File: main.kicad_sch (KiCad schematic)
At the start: 124 parts, among them SW1 SW_Push

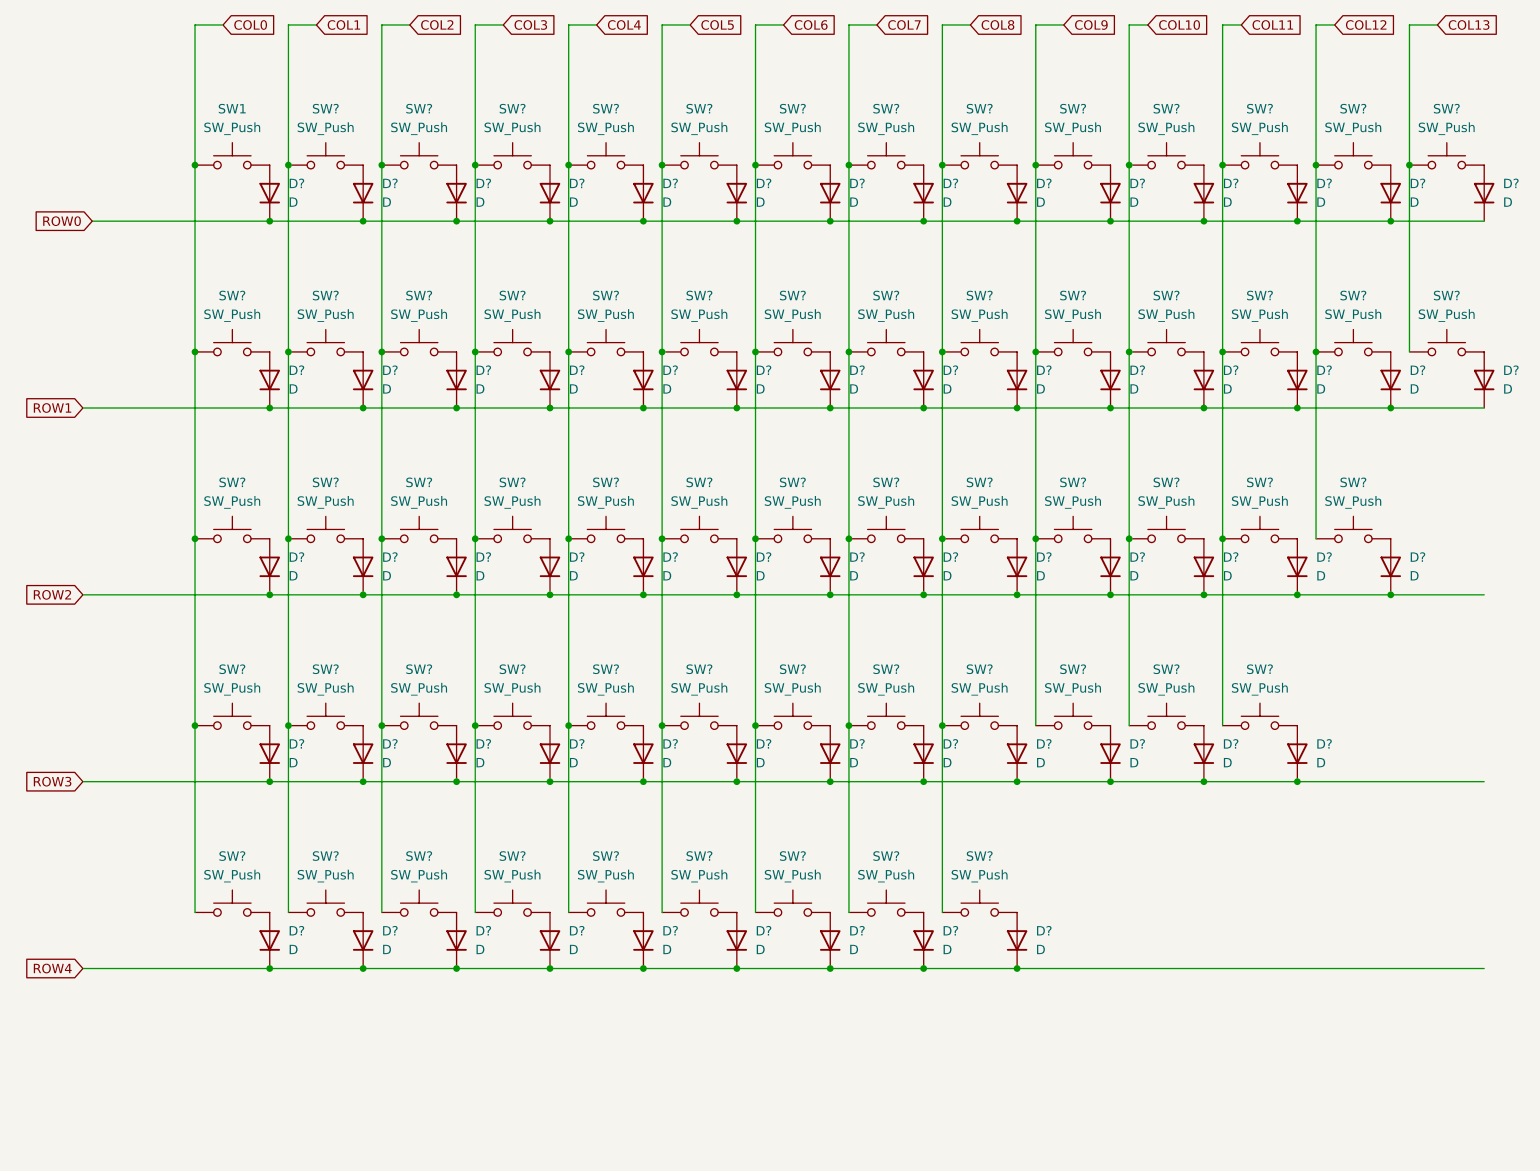
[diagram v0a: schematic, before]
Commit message: Finalilize the Keybord Shematic
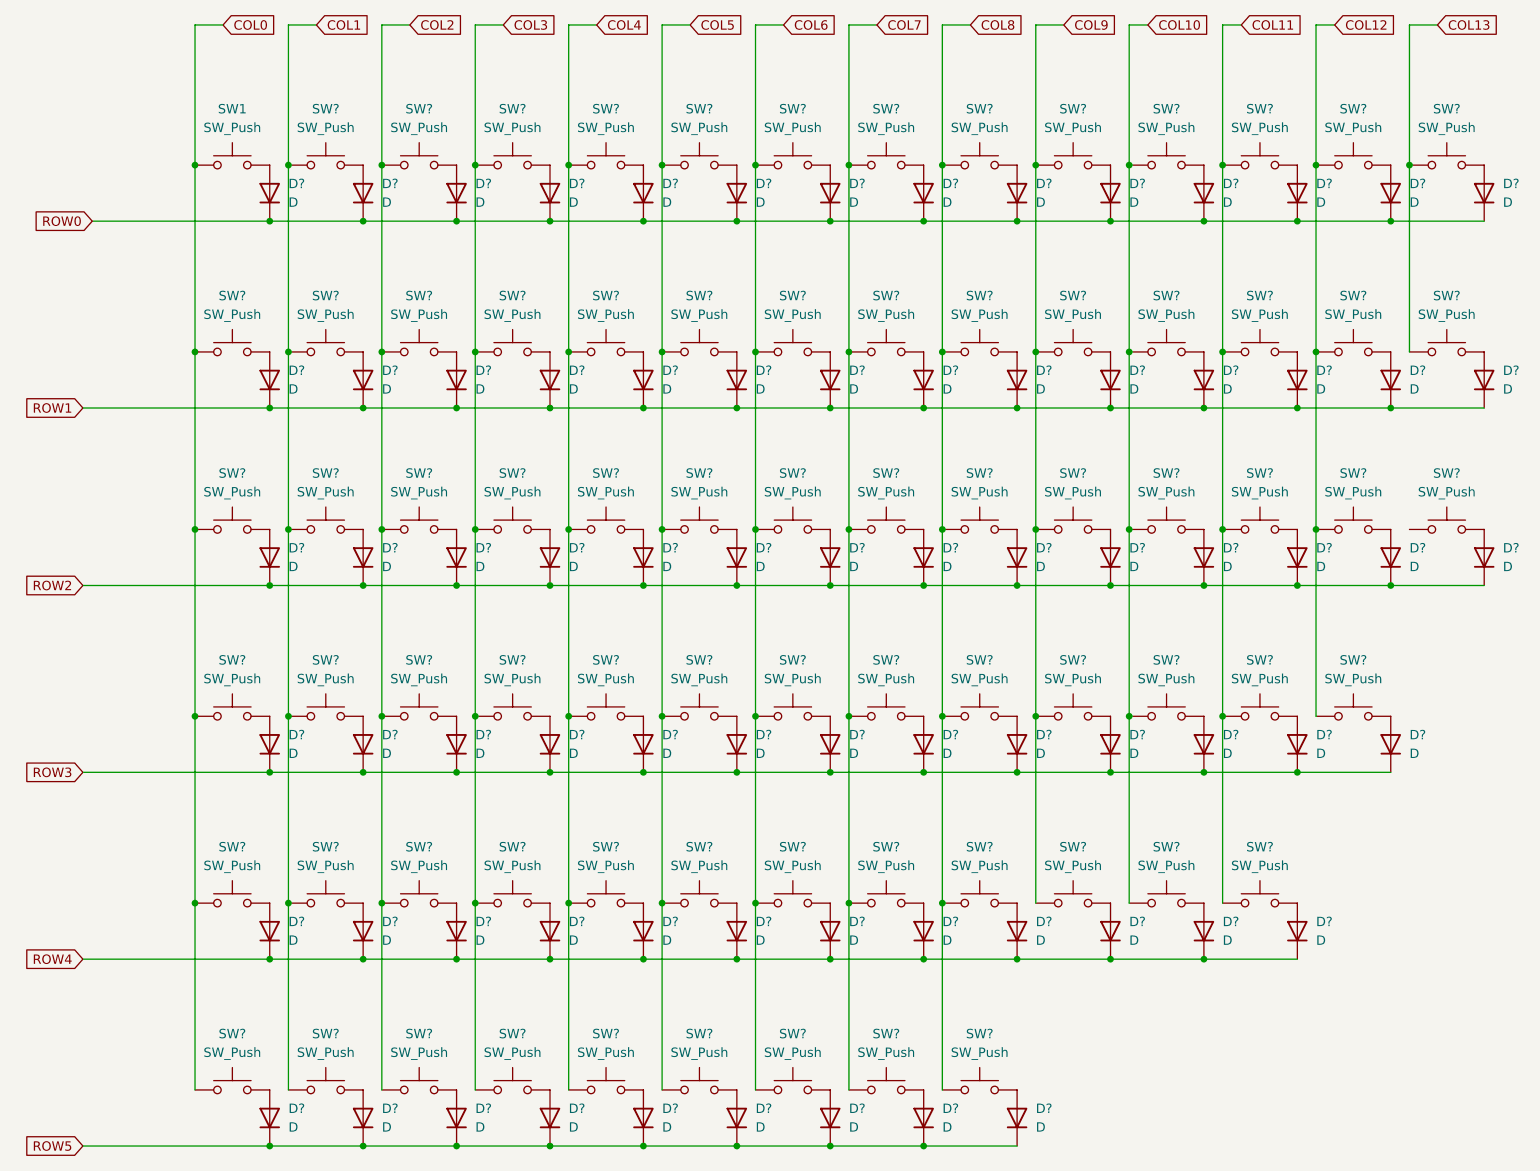
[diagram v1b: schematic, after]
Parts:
- added D? (x14): D, symbol Device:D
- added SW? (x14): SW_Push, JonasLib-Git:MX100H, symbol Switch:SW_Push
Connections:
- net COL0: now also SW?.1
- net COL1: now also SW?.1
- net COL10: now also SW?.1
- net COL11: now also SW?.1
- net COL12: now also SW?.1
- net COL2: now also SW?.1
- net COL3: now also SW?.1
- net COL4: now also SW?.1
- net COL5: now also SW?.1
- net COL6: now also SW?.1
- net COL7: now also SW?.1
- net COL8: now also SW?.1
- net COL9: now also SW?.1
- net ROW2: now also D?.1 (K), D?.1 (K), D?.1 (K), D?.1 (K), D?.1 (K), D?.1 (K), D?.1 (K), D?.1 (K), D?.1 (K), D?.1 (K), D?.1 (K), D?.1 (K), D?.1 (K), D?.1 (K); no longer D?.1 (K), D?.1 (K), D?.1 (K), D?.1 (K), D?.1 (K), D?.1 (K), D?.1 (K), D?.1 (K), D?.1 (K), D?.1 (K), D?.1 (K), D?.1 (K), D?.1 (K)
- net ROW3: now also D?.1 (K), D?.1 (K), D?.1 (K), D?.1 (K), D?.1 (K), D?.1 (K), D?.1 (K), D?.1 (K), D?.1 (K), D?.1 (K), D?.1 (K), D?.1 (K), D?.1 (K); no longer D?.1 (K), D?.1 (K), D?.1 (K), D?.1 (K), D?.1 (K), D?.1 (K), D?.1 (K), D?.1 (K), D?.1 (K), D?.1 (K), D?.1 (K), D?.1 (K)
- net ROW4: now also D?.1 (K), D?.1 (K), D?.1 (K), D?.1 (K), D?.1 (K), D?.1 (K), D?.1 (K), D?.1 (K), D?.1 (K), D?.1 (K), D?.1 (K), D?.1 (K); no longer D?.1 (K), D?.1 (K), D?.1 (K), D?.1 (K), D?.1 (K), D?.1 (K), D?.1 (K), D?.1 (K), D?.1 (K)
- new net: D?.2 (A), SW?.2 (x14)
- new net ROW5: D?.1 (K), D?.1 (K), D?.1 (K), D?.1 (K), D?.1 (K), D?.1 (K), D?.1 (K), D?.1 (K), D?.1 (K)
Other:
- moved on the sheet: D?, SW?
